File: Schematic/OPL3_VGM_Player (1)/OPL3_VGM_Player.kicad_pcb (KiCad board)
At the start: 2 copper layers, 58 parts, among them J1 USB_OTG, J2 Conn_02x03_Odd_Even, J3 Micro_SD_Card, J4 Conn_01x04, J5 Audio-Jack-3, SW1 SW_Push_Dual, SW2 SW_Push_Dual, SW3 SW_Push_Dual, SW4 SW_Push_Dual, SW5 SW_Push_Dual, U1 LD1117S33TR_SOT223, U2 STM32F103C8Tx, U3 CH340E, U4 YMF262-M, U5 YAC512-M, U6 TL074, Y1 8MHz

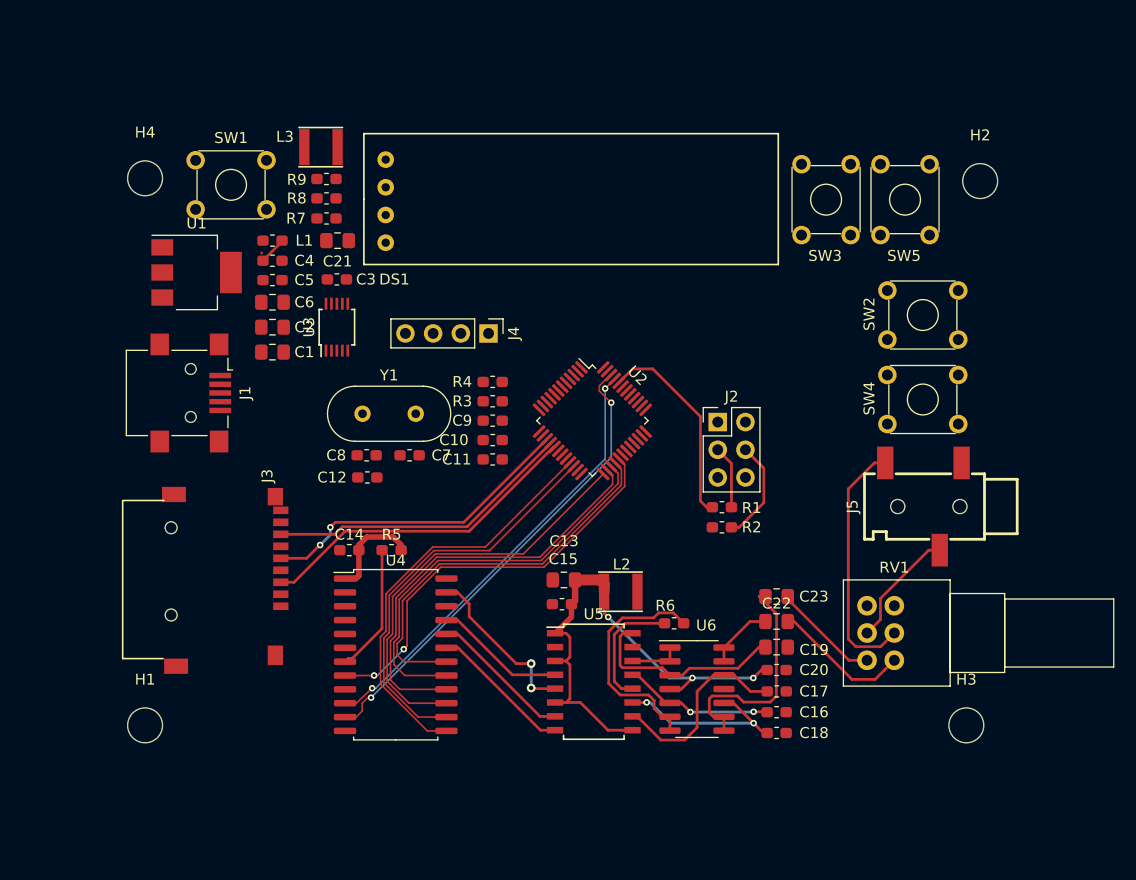
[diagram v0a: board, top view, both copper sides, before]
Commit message: added bom and finished board
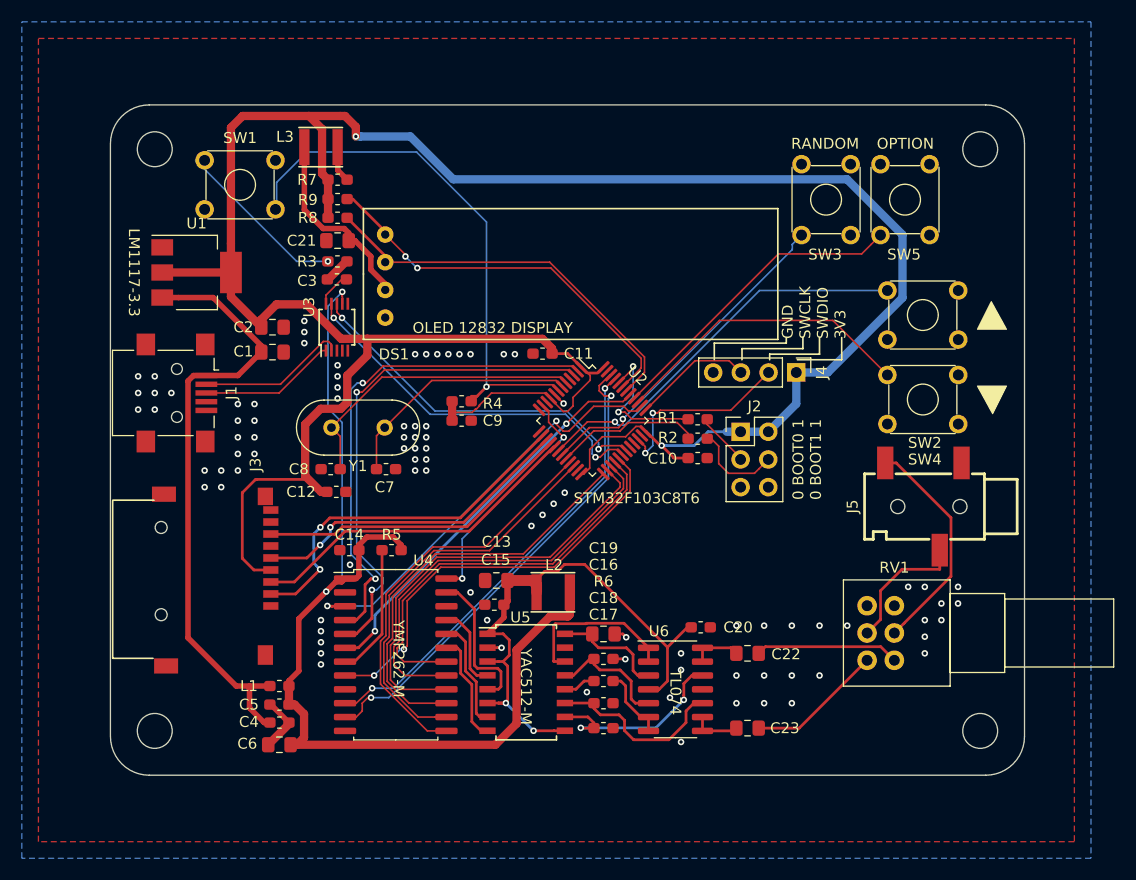
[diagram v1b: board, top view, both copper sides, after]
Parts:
- moved C4 42.4 mm to (104.9, 118.6)
- moved L1 40.8 mm to (104.9, 115.3), turned to 180 degrees
- moved C6 40.6 mm to (104.9, 120.7), turned to 180 degrees
- moved C5 38.9 mm to (104.9, 117.0), turned to 180 degrees
- moved J4 28.4 mm to (152.3, 86.5)
- moved R3 19.2 mm to (110.2, 76.3)
- moved C10 18.9 mm to (143.3, 94.4)
- moved C16 16.6 mm to (134.6, 112.8)
- moved C17 16.2 mm to (134.6, 119.1)
- moved C18 16.1 mm to (134.6, 116.8)
- moved C19 15.9 mm to (134.6, 110.5)
- moved C23 12.4 mm to (147.8, 119.1)
- moved C11 10.7 mm to (129.0, 84.8), turned to 180 degrees
- moved R2 8.43 mm to (143.3, 92.6)
- moved R6 8.37 mm to (134.6, 114.8)
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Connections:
- J1 pad 6: Net-(J1-Pad6) -> GND
- J3 pad : (no net) -> GND
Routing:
- net +3V3: track 0.00 -> 242.7 mm, vias 0 -> 2
- net +5V: track 9.16 -> 94.8 mm, vias 0 -> 2
- net VCC: track 2.57 -> 56.7 mm
- net Net-(R4-Pad2): track 0.00 -> 49.3 mm, vias 0 -> 1
- net YM_A1: track 0.00 -> 46.4 mm, vias 0 -> 2
- net YM_A0: track 0.00 -> 46.0 mm, vias 0 -> 2
- net YM_IC: track 0.00 -> 39.4 mm, vias 0 -> 2
- net YM_WR: track 0.00 -> 36.7 mm, vias 0 -> 2
- net SCL: track 0.00 -> 36.7 mm
- net SDA: track 0.00 -> 36.6 mm, vias 0 -> 2
- net PREV: track 0.00 -> 36.5 mm, vias 0 -> 1
- net RX: track 0.00 -> 34.4 mm, vias 0 -> 2
- net SD_CS: track 0.00 -> 33.7 mm, vias 0 -> 2
- net TX: track 0.00 -> 33.2 mm, vias 0 -> 2
- net RAND: track 0.00 -> 30.8 mm, vias 0 -> 1
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- added copper zone on B.Cu, net GND
- added copper zone on F.Cu, net GND
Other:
- board outline added: 83.8 x 61.5 mm
- board text added: "0 BOOT0 1 0 BOOT1 1"
- board text added: "GND SWCLK SWDIO 3V3"
- board text added: "LM1117-3.3"
- board text added: "OLED 12832 DISPLAY"
- board text added: "OPTION"
- board text added: "RANDOM"
- board text added: "STM32F103C8T6"
